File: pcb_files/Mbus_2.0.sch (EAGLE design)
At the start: 50 parts, among them IC1 NCP1117ST50T3G, IC3 ATMEGA2560-16AU, IC4 RTC_PCF8523T, J1 F-1X18-SIP-100-32Y, J2 USB_A_SMT_FEMALE, Q1 BSS138, Q2 32.768, Q3 BSS138, T1 2N3904, Y1 CSTCE16M0V53-R0 16MHZ

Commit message: 328
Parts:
- removed C3, C4, C5, C6: 100n, SmartPrj:C-EU0603-RND
- removed IC3: ATMEGA2560-16AU, SmartPrj:ATMEGA25602560-16AU
- removed ICSP: 3x2M, SmartPrj:PINHD-2X3
- added C7: 100n, rcl:C-EU
- added ICSP1: ICSP, pinhead:PINHD-2X3
- added Q5: BSS138, adafruit:MOSFET-NREFLOW
- added R18: 10k, SmartPrj:R-EU_R0603
- added R19: 1M, SmartPrj:R-EU_R0603
- added U1: ATMEGA328P-AU, Atmel-ATMEGA328P-AU:ATMEGA328P-AU
- R1: value 1M -> 10k
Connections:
- removed net AREF: C3.1, IC3.AREF
- removed net PB2: IC3.(MOSI/PCINT2)PB2, ICSP.4
- removed net PB3: IC3.(MISO/PCINT3)PB3, ICSP.1
- removed net PB4: IC3.(OC2A/PCINT4)PB4
- removed net PB5: IC3.(OC1A/PCINT5)PB5
- removed net PB6: IC3.(OC1B/PCINT6)PB6
- removed net PB7: IC3.(OC0A/OC1C/PCINT7)PB7, R9.2
- removed net PC4: IC3.(A12)PC4, LCD1.E
- removed net PC6: IC3.(A14)PC6
- removed net PL3: IC3.PL3(OC5A)
- removed net RXD0: IC3.(RXD0/PCIN8)PE0, Q1.D, R2.1
- removed net RXD1: IC3.(RXD1/INT2)PD2, TESTPIN.4
- removed net RXD3: IC3.PJ0(RXD3/PCINT9), J1.7
- removed net TXD0: IC3.(TXD0)PE1, Q3.D, R14.1
- removed net TXD1: IC3.(TXD1/INT3)PD3, TESTPIN.3
- removed net TXD3: IC3.PJ1(TXD3/PCINT10), J1.6
- removed net XTAL1: IC3.XTAL1, R1.1, Y1.3
- removed net XTAL2: IC3.XTAL2, R1.2, Y1.1
- new net CGND: C7.2, U1.GND
- new net MISO: ICSP1.1, Q1.D, R2.1, U1.PB4
- new net MOSI: ICSP1.4, Q3.D, R14.1, U1.PB3
- new net N$13: R19.2, U1.PB6, Y1.1
- new net N$15: PIHEADER.SCLK/GP11, Q5.S, R18.1
- new net PB0: LCD1.E, U1.PB0
- new net PD2: LCD1.DB7, TESTPIN.5, U1.PD2
- new net PD3: LCD1.DB6, TESTPIN.6, U1.PD3
- new net RX: J1.7, TESTPIN.4, U1.PD0
- new net SCLK: ICSP1.3, Q5.D, R1.1, U1.PB5
- new net SS: U1.PB2
- new net TX: J1.6, TESTPIN.3, U1.PD1
- net +3V3: now also Q5.G, R18.2; no longer R7.1, SJ3.2, SJ4.2
- net +5V: now also C7.1, ICSP1.2, R1.2, R7.1, SJ3.2, SJ4.2, U1.AVCC; no longer C4.1, C5.1, C6.1, IC3.AVCC, ICSP.2
- net GND: now also ICSP1.6, POWER.8; no longer C3.2, C4.2, C5.2, C6.2, IC3.AGND, ICSP.6
- net N$1: now also R19.1, U1.PB7, Y1.3; no longer IC3.PK7(ADC15/PCINT23), R16.1
- net N$12: now also PIHEADER.COPI/GP10; no longer PIHEADER.RXI/GP15
- net N$5: now also PIHEADER.CIPO/GP9; no longer PIHEADER.TXO/GP14
- net PB1: now also LCD1.RS, U1.PB1; no longer IC3.(SCK/PCINT1)PB1, ICSP.3
- net PC0: now also U1.PC0; no longer IC3.(A8)PC0, LCD1.DB7
- net PC1: now also U1.PC1; no longer IC3.(A9)PC1, LCD1.DB6
- net PC2: now also U1.PC2; no longer IC3.(A10)PC2, LCD1.DB5
- net PC3: now also U1.PC3; no longer IC3.(A11)PC3, LCD1.DB4
- net PC5: now also J1.5; no longer IC3.(A13)PC5, LCD1.RS
- net PD4: now also LCD1.DB5, TESTPIN.7, U1.PD4; no longer IC3.(ICP1)PD4, TESTPIN.5
- net PD5: now also LCD1.DB4, TESTPIN.8, U1.PD5; no longer IC3.(XCK1)PD5, TESTPIN.6
- net PD6: now also R16.1, U1.PD6; no longer IC3.(T1)PD6, TESTPIN.7
- net PD7: now also R9.2, U1.PD7; no longer IC3.(T0)PD7, J1.5, TESTPIN.8
- net RESET: now also ICSP1.5, U1.PC6; no longer IC3.RESET, ICSP.5
- net SCL: now also U1.PC5; no longer IC3.(SCL/INT0)PD0
- net SDA: now also U1.PC4; no longer IC3.(SDA/INT1)PD1
- net VIN: no longer POWER.8
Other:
- note removed: "(MISO)"
- note removed: "(MOSI)"
- note removed: "(SCK)"
- note removed: "pwm"
- moved on the sheet: C2, D1, IC1, J1, J2, J3, PC1, PC2, Q1, Q3, R1, R14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

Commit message: board 2.0
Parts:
- removed C1: 22p, SmartPrj:C-EU0603-RND
- removed D3: CD1206-S01575, diode:DIODE-MINIMELF
- removed Q5: BSS138, adafruit:MOSFET-NREFLOW
- removed R10, R11, R12, R18: 10k, SmartPrj:R-EU_R0603
- removed R19: 1M, SmartPrj:R-EU_R0603
- removed RESET: TS42031-160R-TR-7260, SmartPrj:TS42
- removed Y1: CSTCE16M0V53-R0 16MHZ, SmartPrj:RESONATORMU
- added C3, C4, C5: 0.1uF, SparkFun:CAP0805
- added C6: (no value), rcl:C-USC0805
- added Q4: CSM-7X-DU, crystal:CSM-7X-DU
- added S2: Reset, SparkFun:TAC_SWITCHSND
- C7: value 100n -> (none); device rcl:C-EU -> rcl:C-USC0805
- R1: value 10k -> 10K; device SmartPrj:R-EU_R0603 -> SparkFun:RESISTOR
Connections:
- removed net CGND: C7.2, U1.GND
- removed net N$12: PIHEADER.COPI/GP10, Q3.S, R15.1
- removed net N$15: PIHEADER.SCLK/GP11, Q5.S, R18.1
- removed net N$5: PIHEADER.CIPO/GP9, Q1.S, R3.1
- new net N$14: C4.2, U1.AREF
- new net PISCL: PIHEADER.PCM_FS/GP19, Q3.S, R15.1
- new net PISDA: PIHEADER.PCM_CLK/GP18, Q1.S, R3.1
- new net RESET1: C5.1, R1.1, S2.3, S2.4, U1.PC6
- net +3V3: no longer Q5.G, R18.2
- net +5V: now also C3.2, U1.VCC, U1.VCC_2; no longer C7.1, D3.C, R10.1, R11.1, R12.1
- net GND: now also C3.1, C4.1, C6.1, C7.1, S2.1, S2.2, U1.GND, U1.GND_2, U1.GND_3; no longer C1.2, RESET.1, RESET.2, Y1.2
- net MISO: no longer Q1.D, R2.1
- net MOSI: no longer Q3.D, R14.1
- net N$1: now also C6.2, Q4.1; no longer R19.1, Y1.3
- net N$13: now also C7.2, Q4.2; no longer R19.2, Y1.1
- net RESET: now also C5.2; no longer C1.1, D3.A, R10.2, RESET.3, RESET.4, U1.PC6
- net SCL: now also Q3.D, R14.1; no longer R11.2
- net SCLK: no longer Q5.D, R1.1
- net SDA: now also Q1.D, R2.1; no longer R12.2
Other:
- moved on the sheet: C2, C7, D1, IC1, J1, J2, L, ON, PC1, PC2, POWER, Q1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

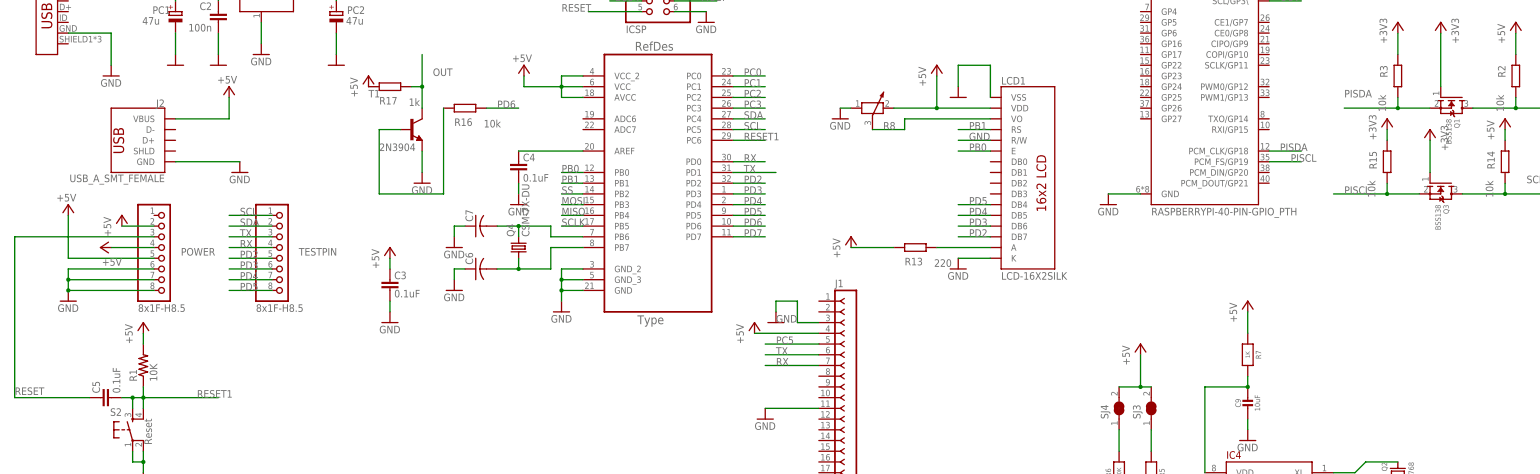
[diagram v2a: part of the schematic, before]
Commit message: pcb layout of 2.0
Signed-off-by: Yiteng Cai <alonsochate@umich.edu>
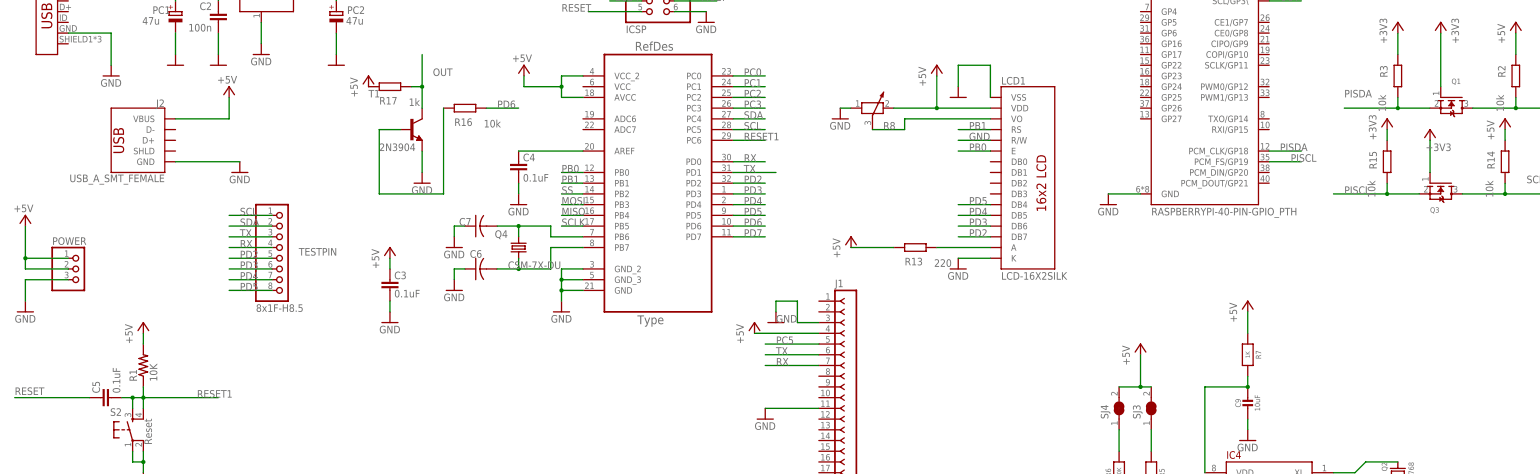
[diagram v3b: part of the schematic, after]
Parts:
- POWER: value 8x1F-H8.5 -> (none); device SmartPrj:PINHD-1X8 -> pinhead:PINHD-1X3
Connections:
- net +5V: now also POWER.1; no longer POWER.4, POWER.5, U1.VCC
- net GND: now also POWER.3; no longer POWER.6, POWER.7, POWER.8
- net RESET: no longer POWER.3
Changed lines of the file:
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@@
 <drawing>
 <settings>
-<setting alwaysvectorfont="no"/>
+<setting alwaysvectorfont="yes"/>
 <setting keepoldvectorfont="yes"/>
 <setting verticaltext="up"/>
@@
 <part name="L" library="led" deviceset="LED" device="CHIP-LED0805" value="YELLOW"/>
 <part name="GND13" library="supply1" deviceset="GND" device=""/>
-<part name="POWER" library="SmartPrj" deviceset="PINHD-1X8" device="" value="8x1F-H8.5"/>
 <part name="PIHEADER" library="SparkFun-Connectors" deviceset="RASPBERRYPI-40-PIN-GPIO" device="_PTH"/>
 <part name="Q2" library="microbuilder" deviceset="CRYSTAL" device="8.0X3.8" value="32.768"/>
@@
 <part name="TESTPIN" library="SmartPrj" deviceset="PINHD-1X8" device="" value="8x1F-H8.5"/>
 <part name="J1" library="con-headers-jp" deviceset="F-1X18-" device="SIP-100-32Y"/>
-<part name="P+18" library="supply1@1" deviceset="+5V" device=""/>
-<part name="P+19" library="supply1@1" deviceset="+5V" device=""/>
 <part name="GND4" library="supply1" deviceset="GND" device=""/>
 <part name="GND6" library="supply1" deviceset="GND" device=""/>
@@
 <part name="T1" library="transistor" library_urn="urn:adsk.eagle:library:402" deviceset="2N3904" device="" package3d_urn="urn:adsk.eagle:package:28523/2"/>
 <part name="C7" library="rcl" deviceset="C-US" device="C0805"/>
+<part name="POWER" library="pinhead" library_urn="urn:adsk.eagle:library:325" deviceset="PINHD-1X3" device="" package3d_urn="urn:adsk.eagle:package:22458/2"/>
 </parts>
 <sheets>
@@
 </plain>
 <instances>
-<instance part="GND5" gate="1" x="17.78" y="50.8" smashed="yes">
-<attribute name="VALUE" x="15.24" y="48.26" size="1.778" layer="96"/>
-</instance>
-<instance part="P+4" gate="1" x="17.78" y="73.66" smashed="yes">
-<attribute name="VALUE" x="19.685" y="76.2" size="1.778" layer="96" rot="R180"/>
+<instance part="GND5" gate="1" x="7.62" y="48.26" smashed="yes">
+<attribute name="VALUE" x="5.08" y="45.72" size="1.778" layer="96"/>
+</instance>
+<instance part="P+4" gate="1" x="7.62" y="71.12" smashed="yes">
+<attribute name="VALUE" x="9.525" y="73.66" size="1.778" layer="96" rot="R180"/>
 </instance>
 <instance part="PC1" gate="G$1" x="43.18" y="119.38" smashed="yes">
@@
 <attribute name="VALUE" x="233.68" y="127" size="1.778" layer="96" rot="R90"/>
 </instance>
-<instance part="POWER" gate="A" x="40.64" y="60.96" smashed="yes">
-<attribute name="NAME" x="44.45" y="61.595" size="1.778" layer="95"/>
-<attribute name="VALUE" x="34.29" y="48.26" size="1.778" layer="96"/>
-</instance>
 <instance part="PIHEADER" gate="G$1" x="287.02" y="104.14" smashed="yes">
 <attribute name="NAME" x="274.32" y="132.842" size="1.778" layer="95"/>
@@
 <attribute name="VALUE" x="199.39" y="2.54" size="1.778" layer="96"/>
 <attribute name="NAME" x="199.39" y="54.102" size="1.778" layer="95"/>
-</instance>
-<instance part="P+18" gate="1" x="30.48" y="71.12" smashed="yes">
-<attribute name="VALUE" x="27.94" y="66.04" size="1.778" layer="96" rot="R90"/>
-</instance>
-<instance part="P+19" gate="1" x="25.4" y="63.5" smashed="yes" rot="R90">
-<attribute name="VALUE" x="30.48" y="60.96" size="1.778" layer="96" rot="R180"/>
 </instance>
 <instance part="GND4" gate="1" x="228.6" y="58.42" smashed="yes">
@@
 </instance>
 <instance part="Q1" gate="G$1" x="345.44" y="99.06" smashed="yes" rot="R270">
-<attribute name="NAME" x="346.075" y="93.98" size="1.27" layer="95" rot="R270"/>
-<attribute name="VALUE" x="344.17" y="93.98" size="1.27" layer="96" rot="R270"/>
+<attribute name="NAME" x="345.44" y="102.235" size="1.27" layer="95"/>
 </instance>
 <instance part="+3V1" gate="G$1" x="342.9" y="116.84" smashed="yes" rot="MR0">
@@
 </instance>
 <instance part="Q3" gate="G$1" x="342.9" y="78.74" smashed="yes" rot="R270">
-<attribute name="NAME" x="343.535" y="73.66" size="1.27" layer="95" rot="R270"/>
-<attribute name="VALUE" x="341.63" y="73.66" size="1.27" layer="96" rot="R270"/>
+<attribute name="NAME" x="340.36" y="71.755" size="1.27" layer="95"/>
 </instance>
 <instance part="P+14" gate="1" x="358.14" y="93.98" smashed="yes">
@@
 </instance>
 <instance part="+3V4" gate="G$1" x="340.36" y="91.44" smashed="yes" rot="MR0">
-<attribute name="VALUE" x="342.9" y="86.36" size="1.778" layer="96" rot="MR90"/>
+<attribute name="VALUE" x="345.44" y="86.36" size="1.778" layer="96" rot="MR0"/>
 </instance>
 <instance part="R2" gate="G$1" x="360.68" y="104.14" smashed="yes" rot="R90">
@@
 </instance>
 <instance part="Q4" gate="P" x="124.46" y="63.5" smashed="yes" rot="R90">
-<attribute name="NAME" x="123.444" y="66.04" size="1.778" layer="95" rot="R90"/>
-<attribute name="VALUE" x="127" y="66.04" size="1.778" layer="96" rot="R90"/>
+<attribute name="NAME" x="121.92" y="67.564" size="1.778" layer="95" rot="R180"/>
+<attribute name="VALUE" x="121.92" y="58.42" size="1.778" layer="96"/>
 </instance>
 <instance part="C6" gate="G$1" x="114.3" y="58.42" smashed="yes" rot="R90">
-<attribute name="NAME" x="113.665" y="59.436" size="1.778" layer="95" rot="R90"/>
+<attribute name="NAME" x="115.824" y="62.865" size="1.778" layer="95" rot="R180"/>
 <attribute name="VALUE" x="118.491" y="59.436" size="1.778" layer="96" rot="R90"/>
 </instance>
@@
 </instance>
 <instance part="C7" gate="G$1" x="114.3" y="68.58" smashed="yes" rot="R90">
-<attribute name="NAME" x="113.665" y="69.596" size="1.778" layer="95" rot="R90"/>
+<attribute name="NAME" x="113.284" y="70.485" size="1.778" layer="95" rot="R180"/>
 <attribute name="VALUE" x="118.491" y="69.596" size="1.778" layer="96" rot="R90"/>
+</instance>
+<instance part="POWER" gate="A" x="20.32" y="58.42" smashed="yes">
+<attribute name="NAME" x="13.97" y="64.135" size="1.778" layer="95"/>
+<attribute name="VALUE" x="13.97" y="50.8" size="1.778" layer="96"/>
 </instance>
 </instances>
@@
 </segment>
 <segment>
-<wire x1="17.78" y1="60.96" x2="17.78" y2="71.12" width="0.1524" layer="91"/>
-<wire x1="38.1" y1="60.96" x2="17.78" y2="60.96" width="0.1524" layer="91"/>
-<pinref part="P+4" gate="1" pin="+5V"/>
-<pinref part="POWER" gate="A" pin="5"/>
-</segment>
-<segment>
 <wire x1="195.58" y1="43.18" x2="180.34" y2="43.18" width="0.1524" layer="91"/>
 <pinref part="P+17" gate="1" pin="+5V"/>
@@
 </segment>
 <segment>
-<pinref part="POWER" gate="A" pin="2"/>
-<wire x1="38.1" y1="68.58" x2="30.48" y2="68.58" width="0.1524" layer="91"/>
-<pinref part="P+18" gate="1" pin="+5V"/>
-</segment>
-<segment>
-<pinref part="POWER" gate="A" pin="4"/>
-<wire x1="38.1" y1="63.5" x2="27.94" y2="63.5" width="0.1524" layer="91"/>
-<pinref part="P+19" gate="1" pin="+5V"/>
-</segment>
-<segment>
 <pinref part="P+13" gate="1" pin="+5V"/>
 <wire x1="55.88" y1="99.06" x2="55.88" y2="93.98" width="0.1524" layer="91"/>
@@
 <wire x1="139.7" y1="99.06" x2="134.62" y2="99.06" width="0.1524" layer="91"/>
 <wire x1="134.62" y1="99.06" x2="134.62" y2="101.6" width="0.1524" layer="91"/>
-<pinref part="U1" gate="A" pin="VCC"/>
-<wire x1="139.7" y1="101.6" x2="134.62" y2="101.6" width="0.1524" layer="91"/>
 <junction x="134.62" y="101.6"/>
 <pinref part="U1" gate="A" pin="VCC_2"/>
@@
 <pinref part="P+15" gate="1" pin="+5V"/>
 </segment>
+<segment>
+<pinref part="POWER" gate="A" pin="2"/>
+<wire x1="17.78" y1="58.42" x2="7.62" y2="58.42" width="0.1524" layer="91"/>
+<pinref part="P+4" gate="1" pin="+5V"/>
+<wire x1="7.62" y1="58.42" x2="7.62" y2="60.96" width="0.1524" layer="91"/>
+<pinref part="POWER" gate="A" pin="1"/>
+<wire x1="7.62" y1="60.96" x2="7.62" y2="68.58" width="0.1524" layer="91"/>
+<wire x1="17.78" y1="60.96" x2="7.62" y2="60.96" width="0.1524" layer="91"/>
+<junction x="7.62" y="60.96"/>
+</segment>
 </net>
 <net name="GND" class="2">
@@
 <pinref part="GND14" gate="1" pin="GND"/>
 <pinref part="ON" gate="G$1" pin="C"/>
-</segment>
-<segment>
-<wire x1="38.1" y1="58.42" x2="17.78" y2="58.42" width="0.1524" layer="91"/>
-<wire x1="17.78" y1="58.42" x2="17.78" y2="55.88" width="0.1524" layer="91"/>
-<wire x1="38.1" y1="55.88" x2="17.78" y2="55.88" width="0.1524" layer="91"/>
-<wire x1="17.78" y1="55.88" x2="17.78" y2="53.34" width="0.1524" layer="91"/>
-<junction x="17.78" y="55.88"/>
-<pinref part="GND5" gate="1" pin="GND"/>
-<pinref part="POWER" gate="A" pin="6"/>
-<pinref part="POWER" gate="A" pin="7"/>
-<pinref part="POWER" gate="A" pin="8"/>
-<wire x1="38.1" y1="53.34" x2="17.78" y2="53.34" width="0.1524" layer="91"/>
-<junction x="17.78" y="53.34"/>
 </segment>
 <segment>
@@
 <wire x1="109.22" y1="68.58" x2="109.22" y2="66.04" width="0.1524" layer="91"/>
 </segment>
+<segment>
+<pinref part="GND5" gate="1" pin="GND"/>
+<wire x1="7.62" y1="50.8" x2="7.62" y2="55.88" width="0.1524" layer="91"/>
+<pinref part="POWER" gate="A" pin="3"/>
+<wire x1="7.62" y1="55.88" x2="17.78" y2="55.88" width="0.1524" layer="91"/>
+</segment>
 </net>
 <net name="RESET" class="0">
 <segment>
-<wire x1="5.08" y1="66.04" x2="38.1" y2="66.04" width="0.1524" layer="91"/>
-<wire x1="5.08" y1="27.94" x2="5.08" y2="66.04" width="0.1524" layer="91"/>
 <label x="5.08" y="28.575" size="1.778" layer="95"/>
-<pinref part="POWER" gate="A" pin="3"/>
 <pinref part="C5" gate="G$1" pin="2"/>
 <wire x1="22.86" y1="27.94" x2="5.08" y2="27.94" width="0.1524" layer="91"/>
